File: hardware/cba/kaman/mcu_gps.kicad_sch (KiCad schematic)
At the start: 45 parts, among them Q1 MMDT5551, Q2 DTC143X, Q3 DTC143X, SW1 SW_Push, SW2 SW_Push, U1 ESP32-C6-MINI-1, U2 L80-R, U3 NEO-M8N, U4 AT24CS64-SSHM, U8 Ai-Thinker-Ra-01

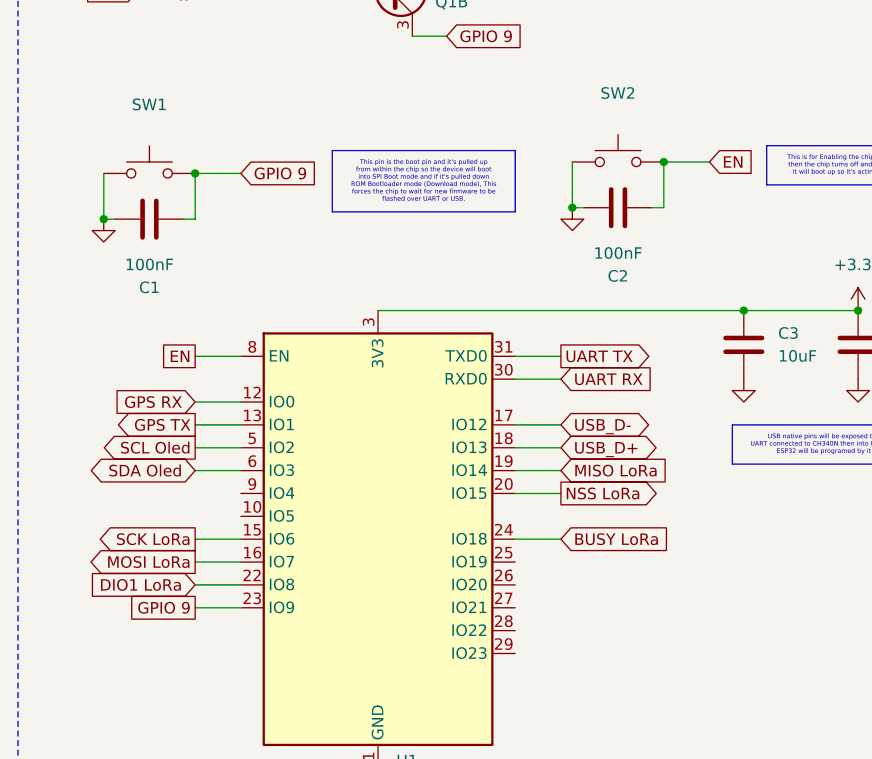
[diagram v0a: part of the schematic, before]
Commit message: hw(pcb): final 0.2v pcb
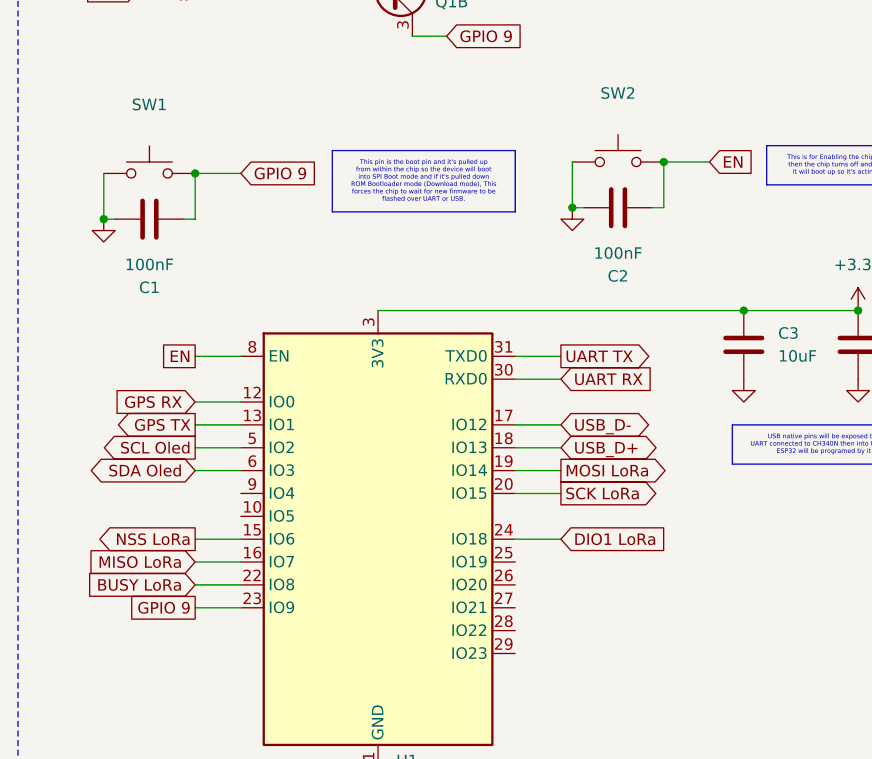
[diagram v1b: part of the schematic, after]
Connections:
- net BUSY LoRa: now also U1.22 (IO8); no longer U1.24 (IO18)
- net DIO1 LoRa: now also U1.24 (IO18); no longer U1.22 (IO8)
- net MISO LoRa: now also U1.16 (IO7); no longer U1.19 (IO14)
- net MOSI LoRa: now also U1.19 (IO14); no longer U1.16 (IO7)
- net NSS LoRa: now also U1.15 (IO6); no longer U1.20 (IO15)
- net SCK LoRa: now also U1.20 (IO15); no longer U1.15 (IO6)
